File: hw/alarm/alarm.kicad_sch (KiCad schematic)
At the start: 50 parts, among them IC1 DS3231S#T&R, IC2 TSOP38238, IC3 SHT40-BD1B-R2, IC4 23K256-I_SN, IC5 PEC11S-929K-S0015, J1 4328, J2 SFV24R-4STBE1HLF, Q1 DMG2305UX-7, Q3 Si1308EDL-T1-GE3, U1 RaspberryPi_Pico, U3 2462, U4 AS1115-BSST, U5 TDCR1060M

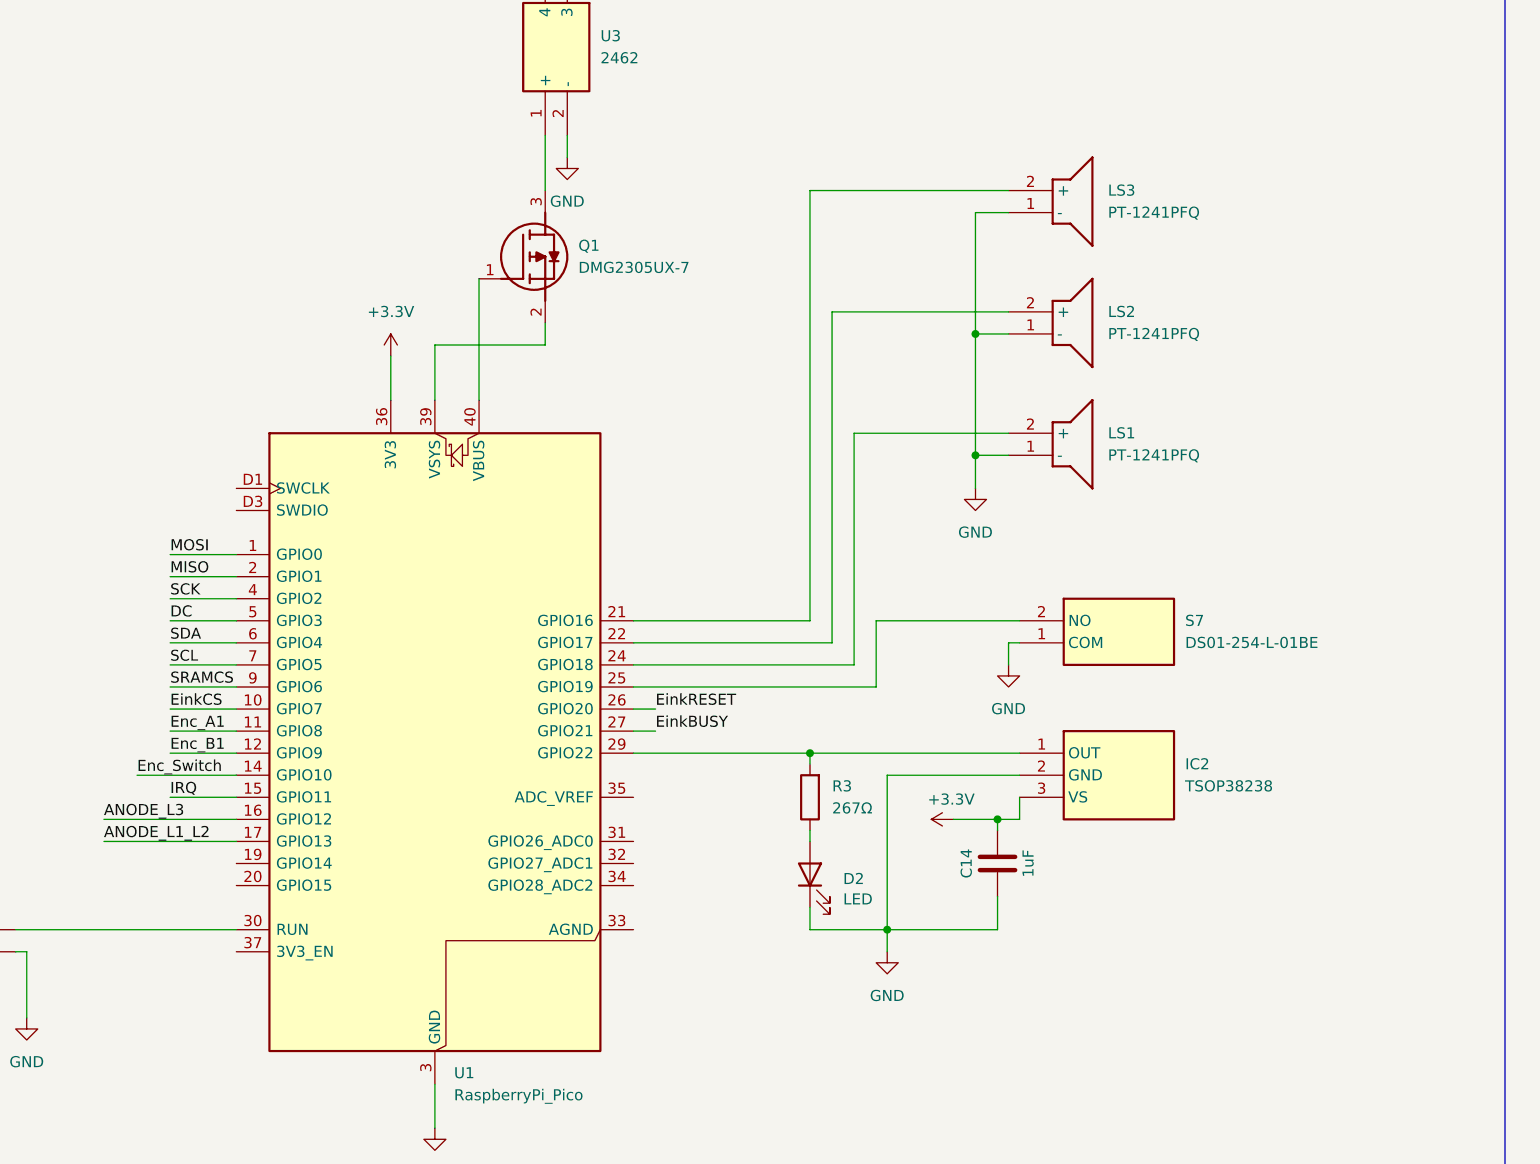
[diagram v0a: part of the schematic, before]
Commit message: Finish board layout initial ver
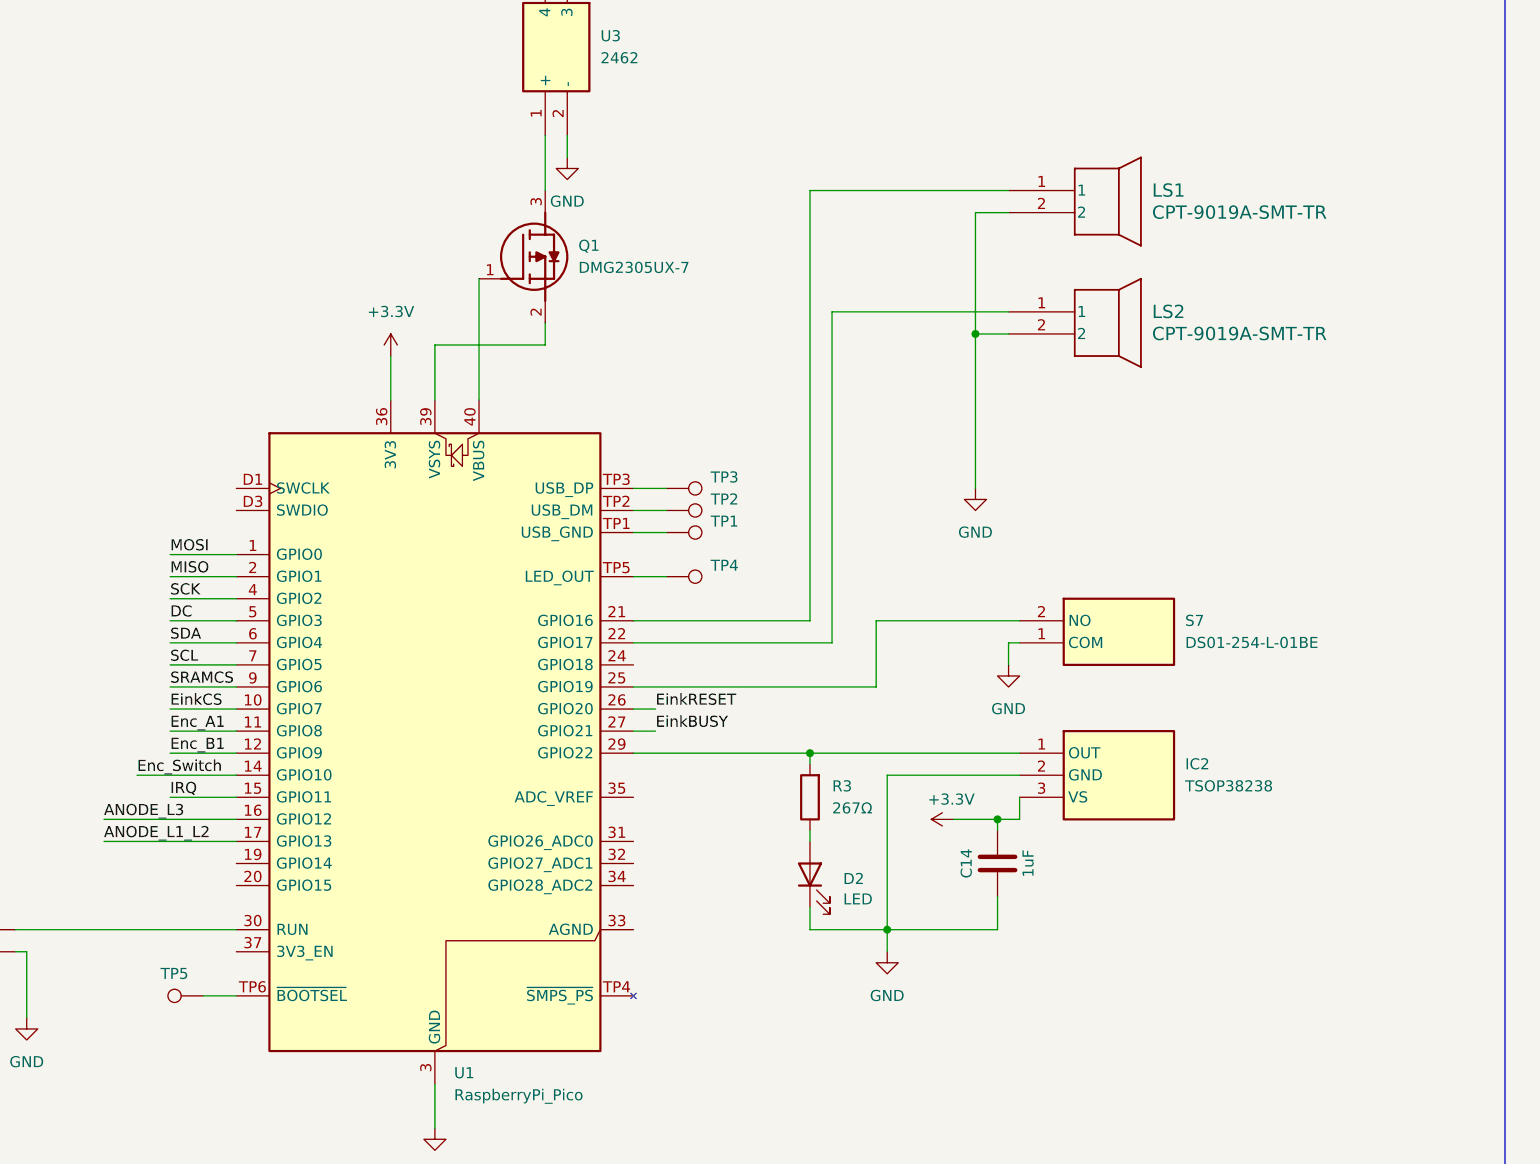
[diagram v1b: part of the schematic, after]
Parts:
- removed LS1, LS2, LS3: PT-1241PFQ, PT1241PFQ, symbol SamacSys_Parts:PT-1241PFQ
- added LS1, LS2: CPT-9019A-SMT-TR, CPT-9019A_CUD, symbol CPT_9019A_SMT_TR:CPT-9019A-SMT-TR
- added TP1, TP2, TP3, TP4, TP5: TestPoint, TestPoint:TestPoint_Pad_1.0x1.0mm, symbol Connector:TestPoint
- U1: footprint Module_RaspberryPi_Pico:RaspberryPi_Pico_Original_SMD_MountingHoles_HandSolder_Castellated -> Module_RaspberryPi_Pico:RaspberryPi_Pico_Original_SMD; symbol MCU_Module_RaspberryPi_Pico:RaspberryPi_Pico_DebugPins -> MCU_Module_RaspberryPi_Pico:RaspberryPi_Pico_SecondaryPins
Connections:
- net GND: now also LS1.2, LS2.2
- net at U1.22 (GPIO17): now also LS2.1
- net at U1.21 (GPIO16): now also LS1.1
- new net: TP2.1, U1.TP2 (USB_DM)
- new net: TP1.1, U1.TP1 (USB_GND)
- new net: TP3.1, U1.TP3 (USB_DP)
- new net: TP4.1, U1.TP5 (LED_OUT)
- new net: TP5.1, U1.TP6 (~{BOOTSEL})
